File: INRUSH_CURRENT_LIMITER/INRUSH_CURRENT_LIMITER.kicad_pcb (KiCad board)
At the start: 2 copper layers, 72 x 20 mm, 7 parts, among them J1 IN, J2 OUT

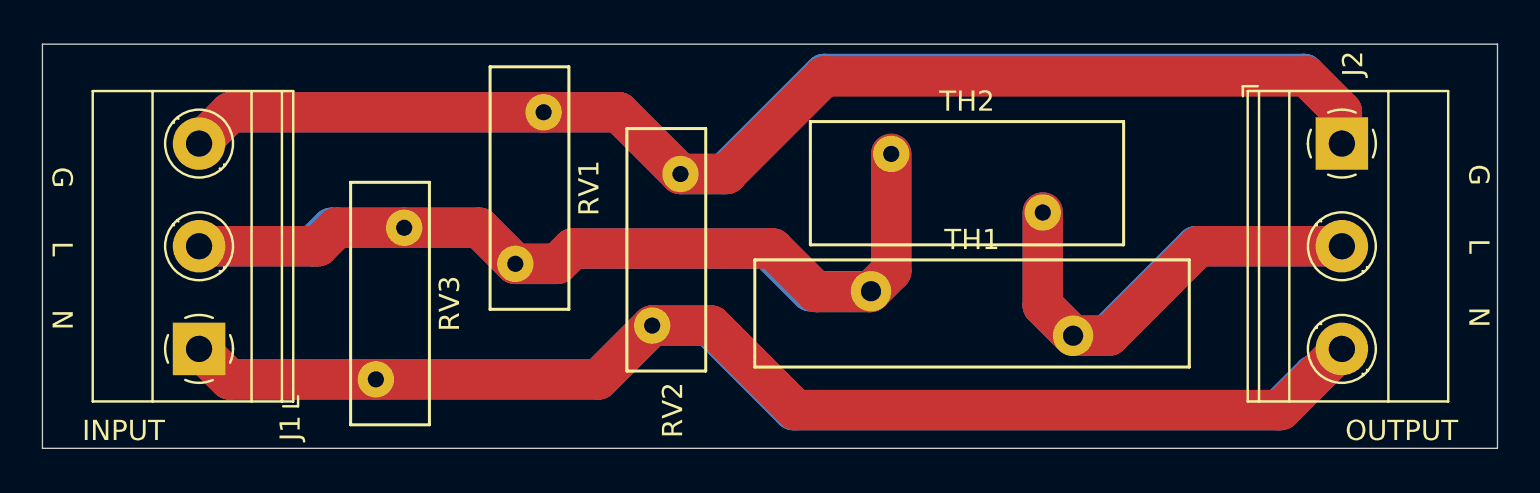
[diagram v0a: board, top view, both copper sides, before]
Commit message: silkscreen labels
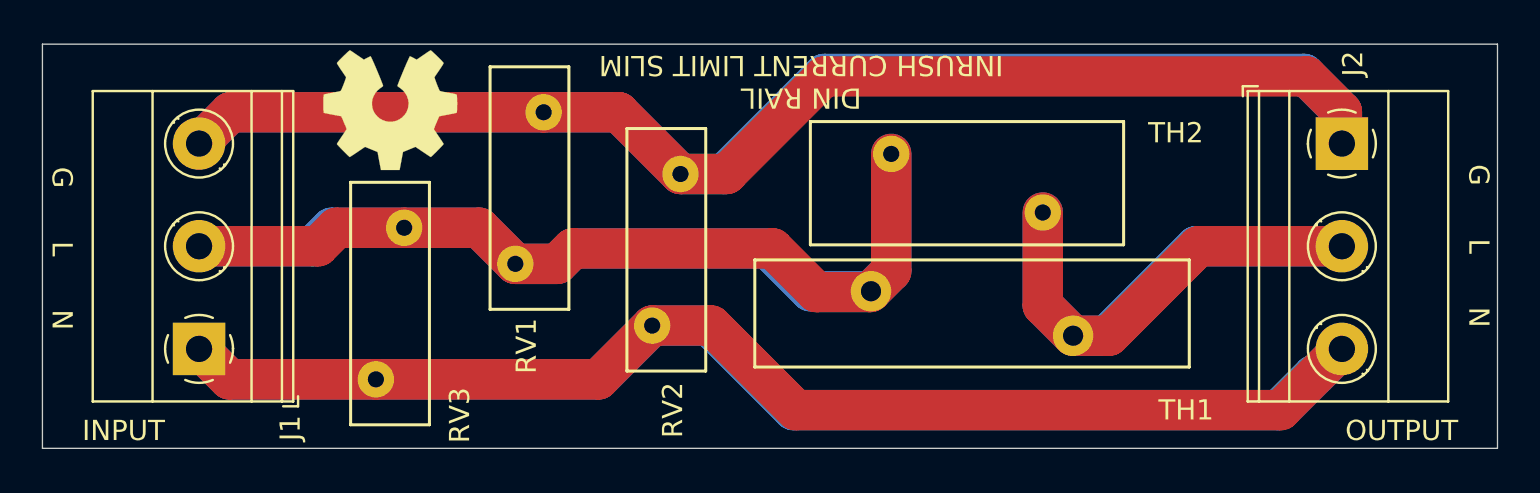
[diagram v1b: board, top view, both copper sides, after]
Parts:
- added REF**: OSHW-Symbol_6.7x6mm_SilkScreen, Symbol:OSHW-Symbol_6.7x6mm_SilkScreen, F.Cu at (117.2, 103.3)
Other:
- board text added: "DIN RAIL INRUSH CURRENT LIMIT SLIM"
